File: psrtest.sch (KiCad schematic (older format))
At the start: 1 part, among them U1 IS66WVE4M16EBLL-70BLI

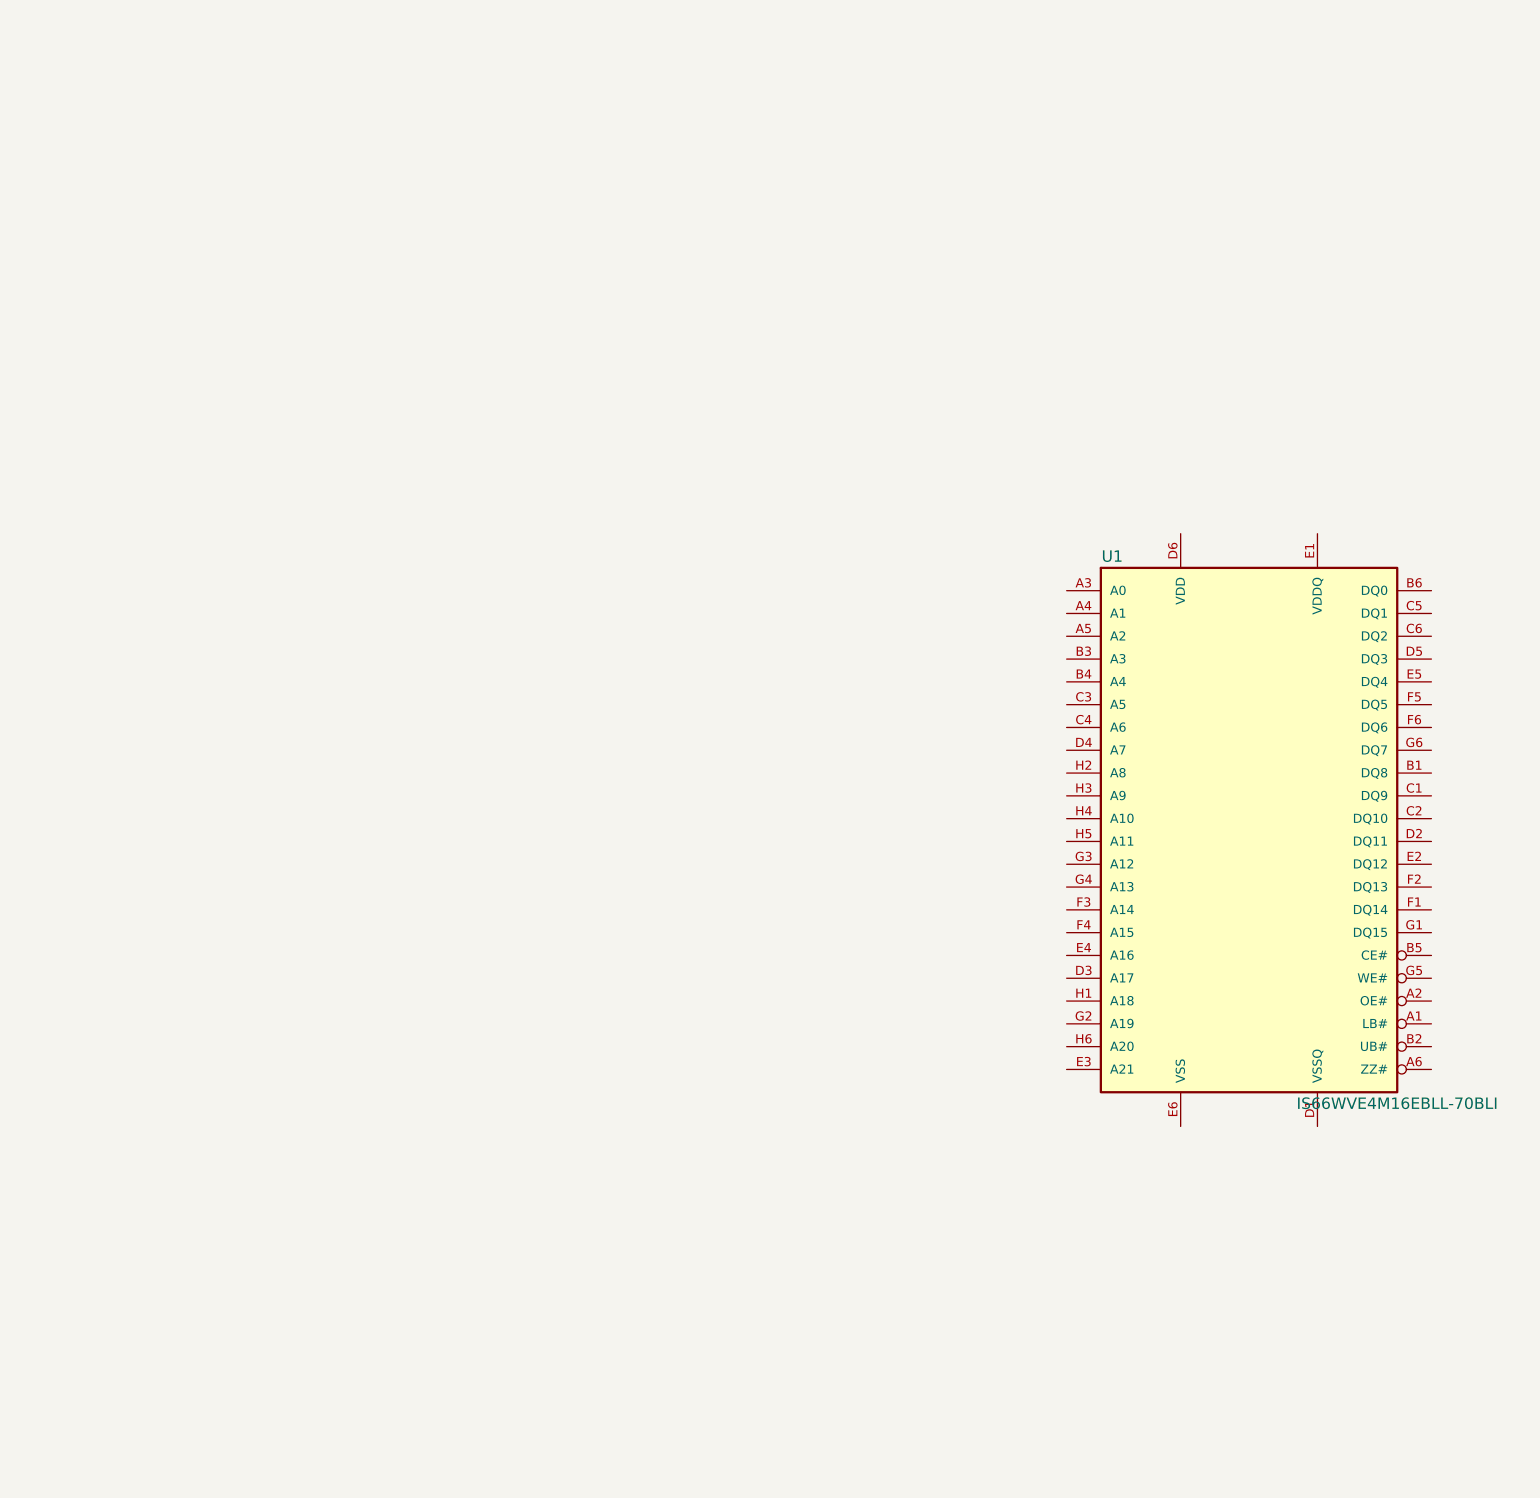
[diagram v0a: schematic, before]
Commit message: Initial fanout.
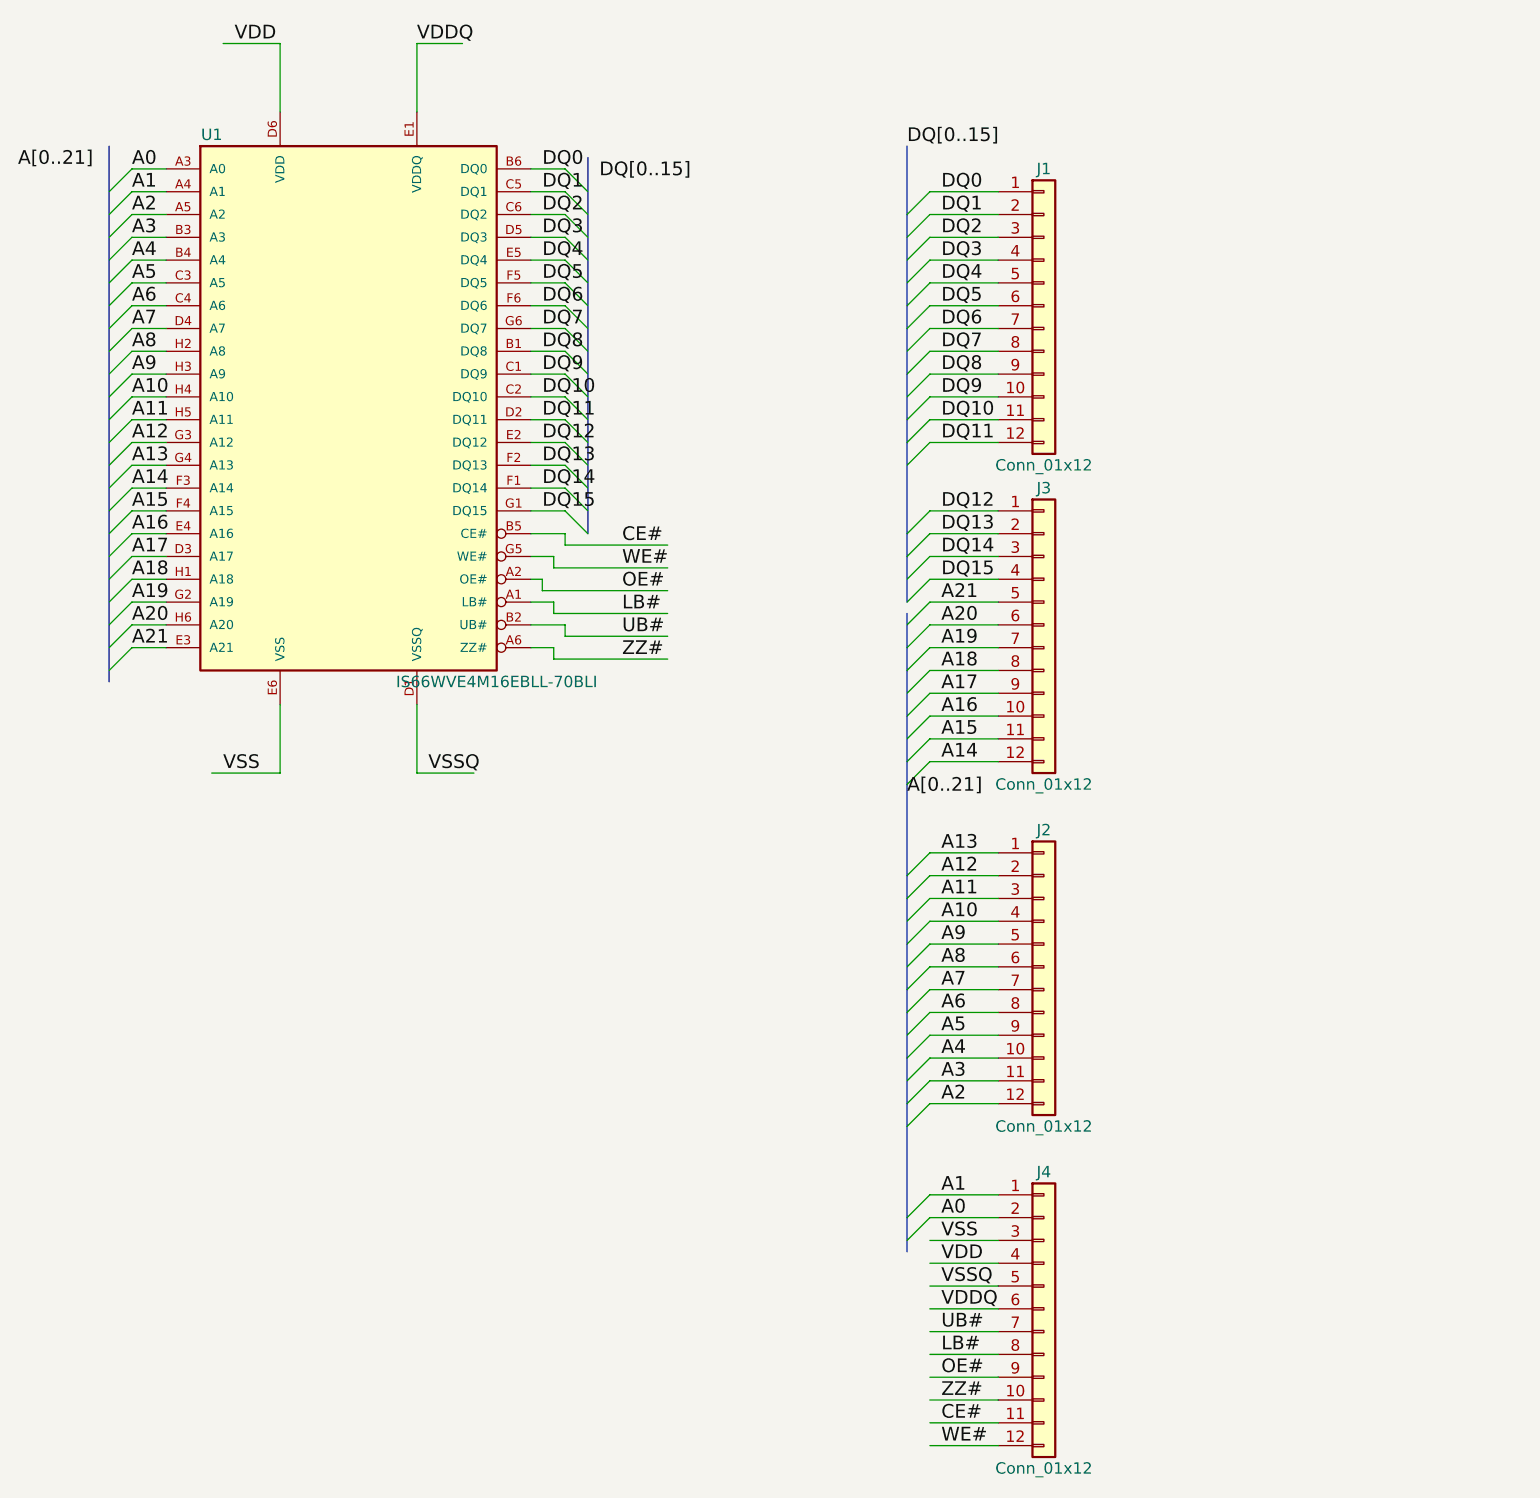
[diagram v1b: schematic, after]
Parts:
- added J1, J2, J3, J4: Conn_01x12, Pin_Headers:Pin_Header_Straight_1x12_Pitch2.54mm, symbol Conn_01x12
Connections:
- net labels added: A0, A1, A10, A11, A12, A13, A14, A15, A16, A17, A18, A19, A2, A20, A21, A3, A4, A5, A6, A7, A8, A9, A[0..21], CE#, DQ0, DQ1, DQ10, DQ11, DQ12, DQ13, DQ14, DQ15, DQ2, DQ3, DQ4, DQ5, DQ6, DQ7, DQ8, DQ9, DQ[0..15], LB#, OE#, UB#, VDD, VDDQ, VSS, VSSQ, WE#, ZZ#
- wire segments 0 -> 112
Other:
- moved on the sheet: U1
